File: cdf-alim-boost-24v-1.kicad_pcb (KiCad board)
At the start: 4 copper layers, 70 x 50 mm, 99 parts, among them J1 Conn_01x02, J2 Conn_01x02, J3 Conn_01x02, Q1 BSC019N04LS, Q2 BSC019N04LS, Q3 BSC019N04LS, Q4 BSC019N04LS, Q5 BSC019N04LS, U1 HT753-1, U2 TPS25983, U4 LM5122

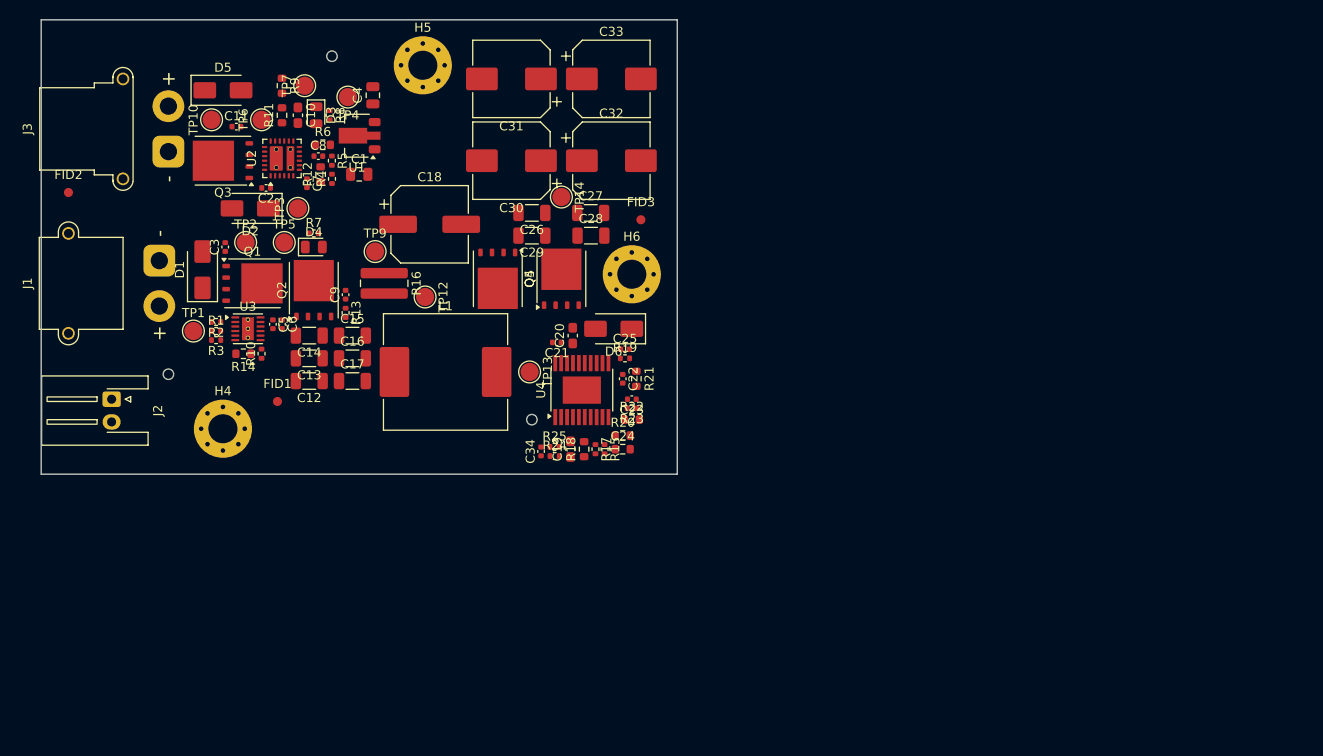
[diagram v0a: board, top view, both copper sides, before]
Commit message: pcb: center board
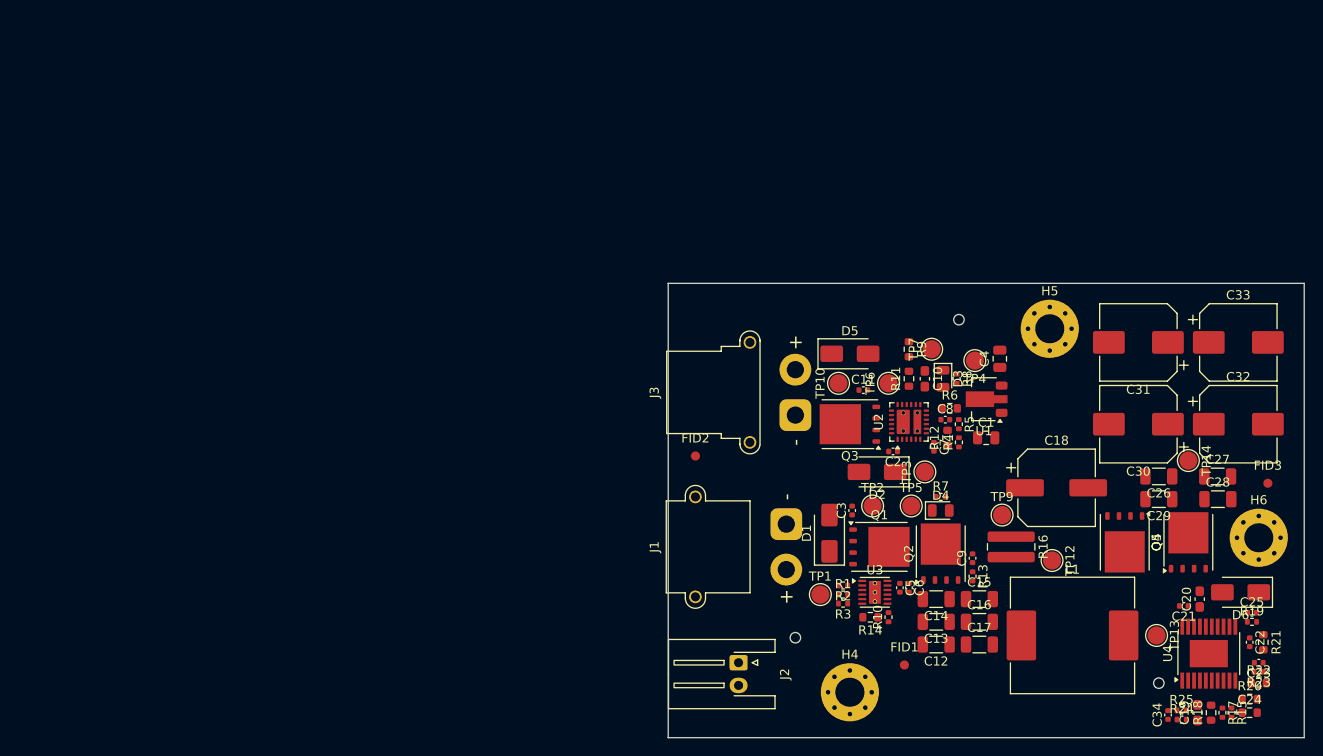
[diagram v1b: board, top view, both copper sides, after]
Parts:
- moved C7 74.8 mm to (144.2, 86.0)
- moved R5 74.8 mm to (147.0, 83.5)
- moved C1 74.8 mm to (150.0, 85.0)
- moved C10 74.8 mm to (143.2, 78.5)
- moved C11 74.8 mm to (136.5, 79.8)
- moved C12 74.8 mm to (144.5, 107.8)
- moved C13 74.8 mm to (144.5, 105.2)
- moved C14 74.8 mm to (144.5, 102.8)
- moved C15 74.8 mm to (149.2, 102.8)
- moved C16 74.8 mm to (149.2, 105.2)
- moved C17 74.8 mm to (149.2, 107.8)
- moved C18 74.8 mm to (157.8, 90.5)
- moved C19 74.8 mm to (173.2, 115.2)
- moved C2 74.8 mm to (139.8, 86.5)
- moved C20 74.8 mm to (173.5, 102.8)
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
